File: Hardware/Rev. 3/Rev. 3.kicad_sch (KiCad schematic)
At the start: 26 parts, among them J1 84952-8, Q1 NMOS, U1 MCP73831-2-OT, U3 W25Q128JVS, U4 LM324

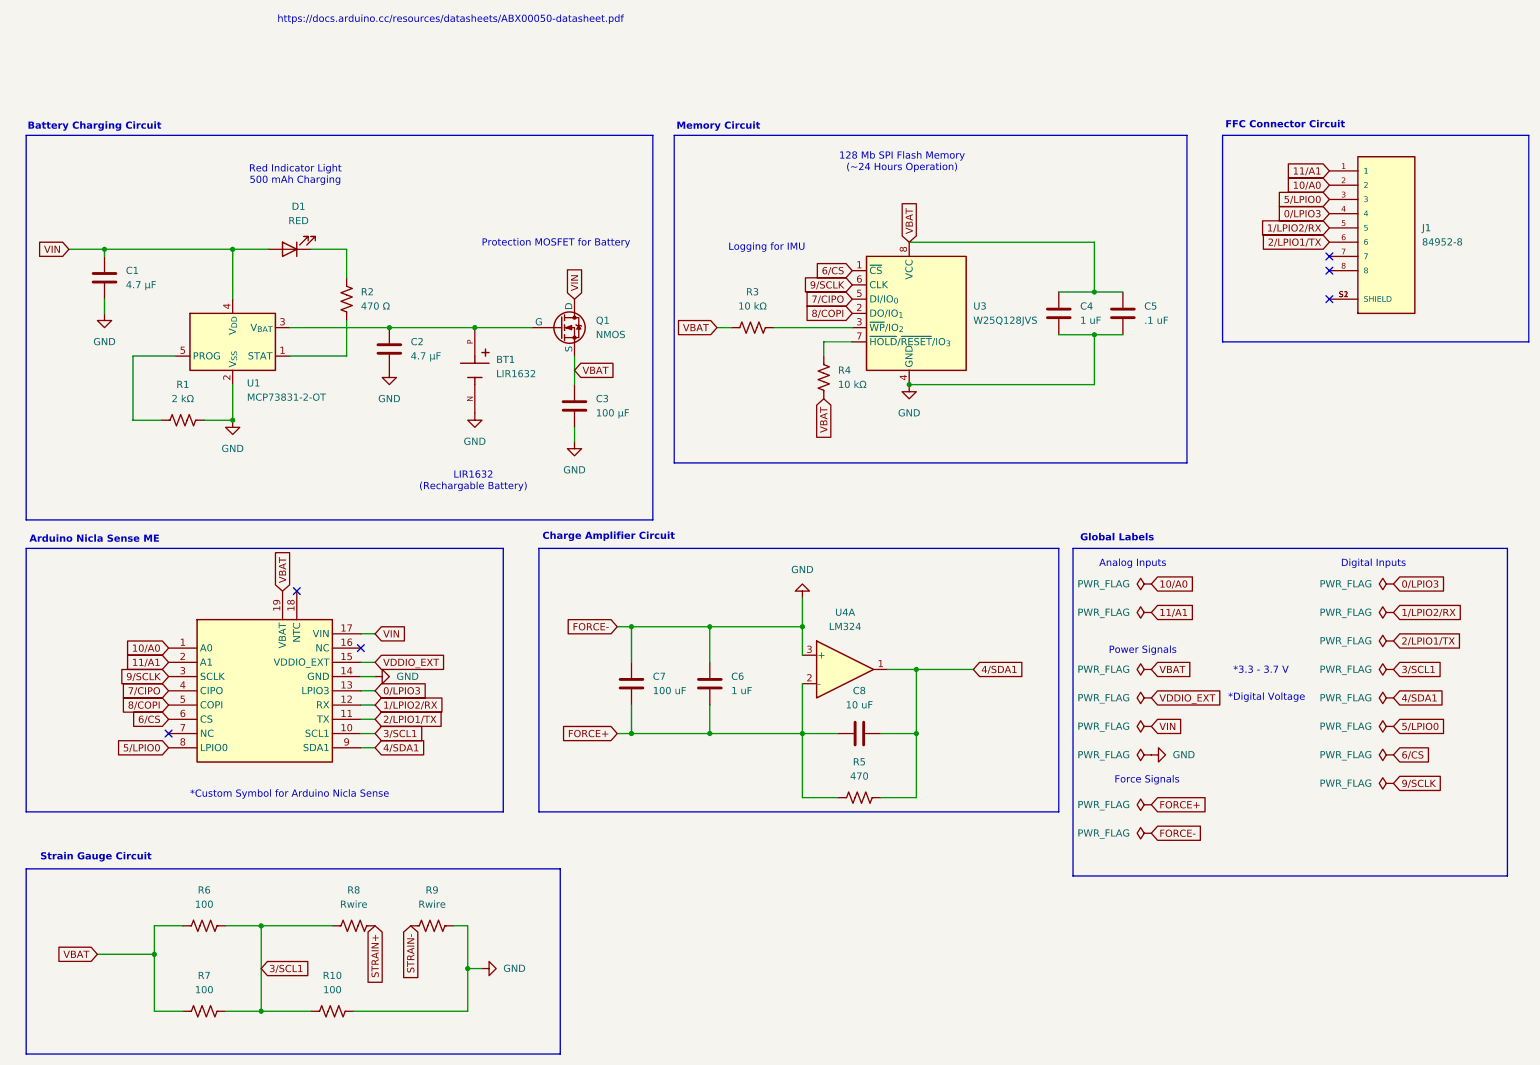
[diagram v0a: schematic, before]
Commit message: Week 13 Changes
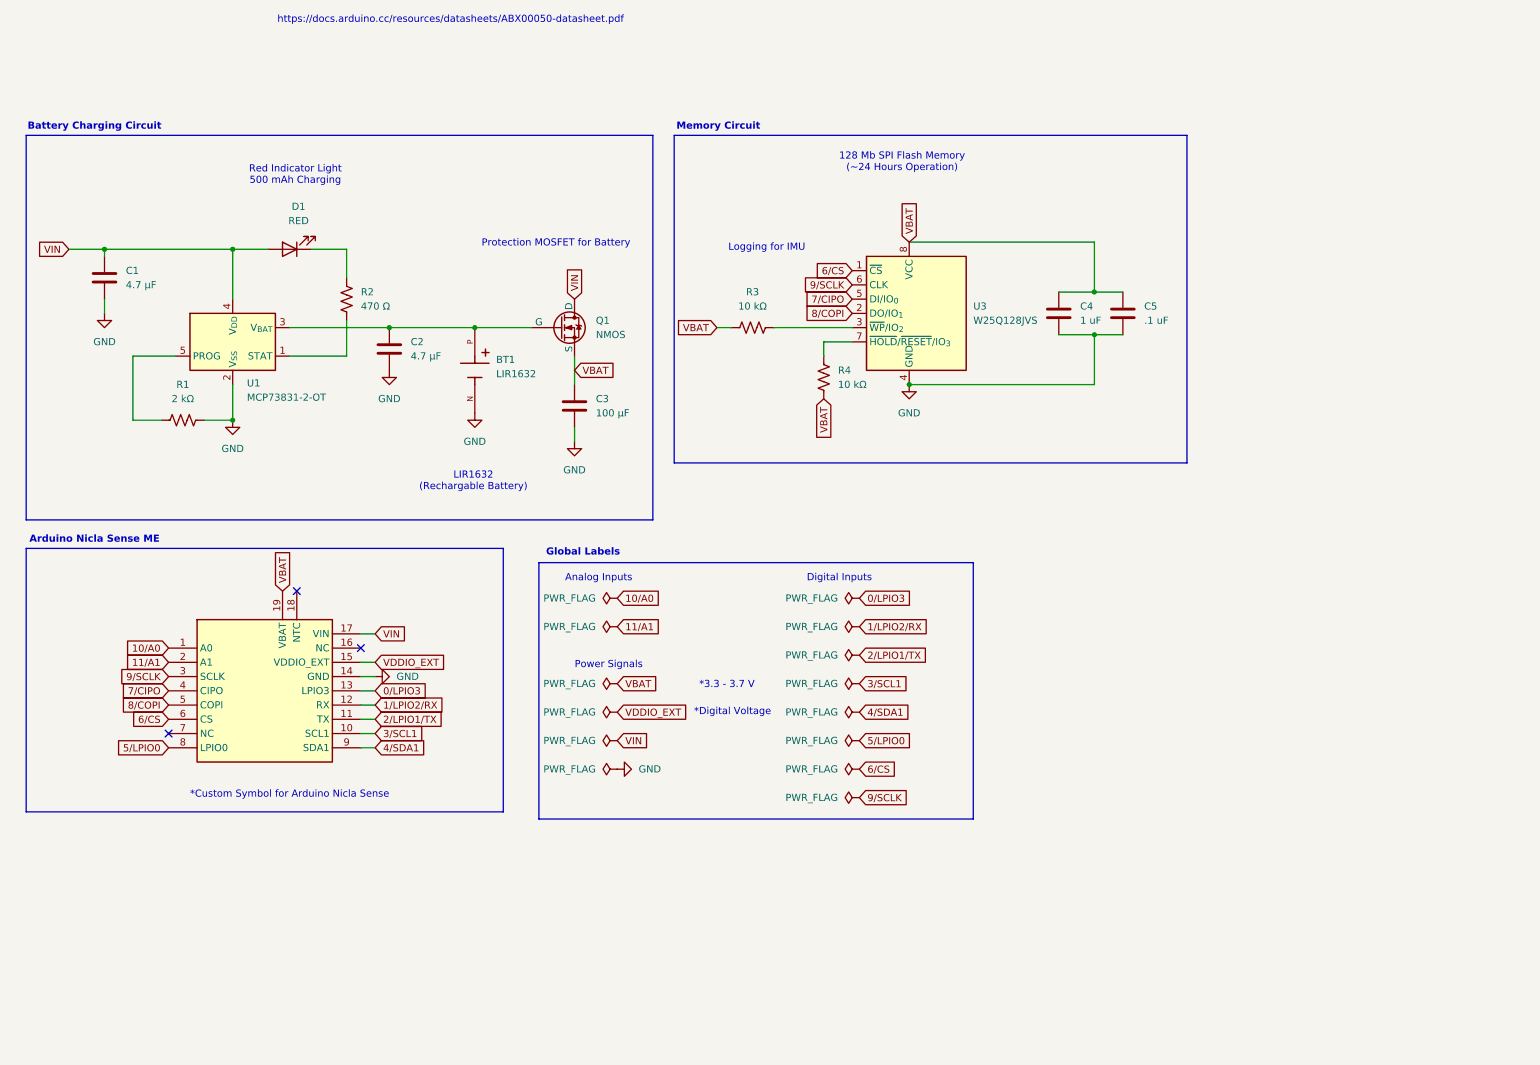
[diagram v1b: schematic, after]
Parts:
- removed C6: 1 uF, symbol Device:C
- removed C7: 100 uF, symbol Device:C
- removed C8: 10 uF, symbol Device:C
- removed J1: 84952-8, footprints:FFC_84952-8, symbol symbols:84952-8
- removed R10, R6, R7: 100, symbol Device:R_US
- removed R5: 470, symbol Device:R_US
- removed R8, R9: Rwire, symbol Device:R_US
- removed U4: LM324, symbol Amplifier_Operational:LM324
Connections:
- no-connect marks 6 -> 3
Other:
- note removed: "Charge Amplifier Circuit"
- note removed: "FFC Connector Circuit"
- note removed: "Force Signals"
- note removed: "Strain Gauge Circuit"
